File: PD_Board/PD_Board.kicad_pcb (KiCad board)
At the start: 2 copper layers, 116 x 63 mm, 12 parts

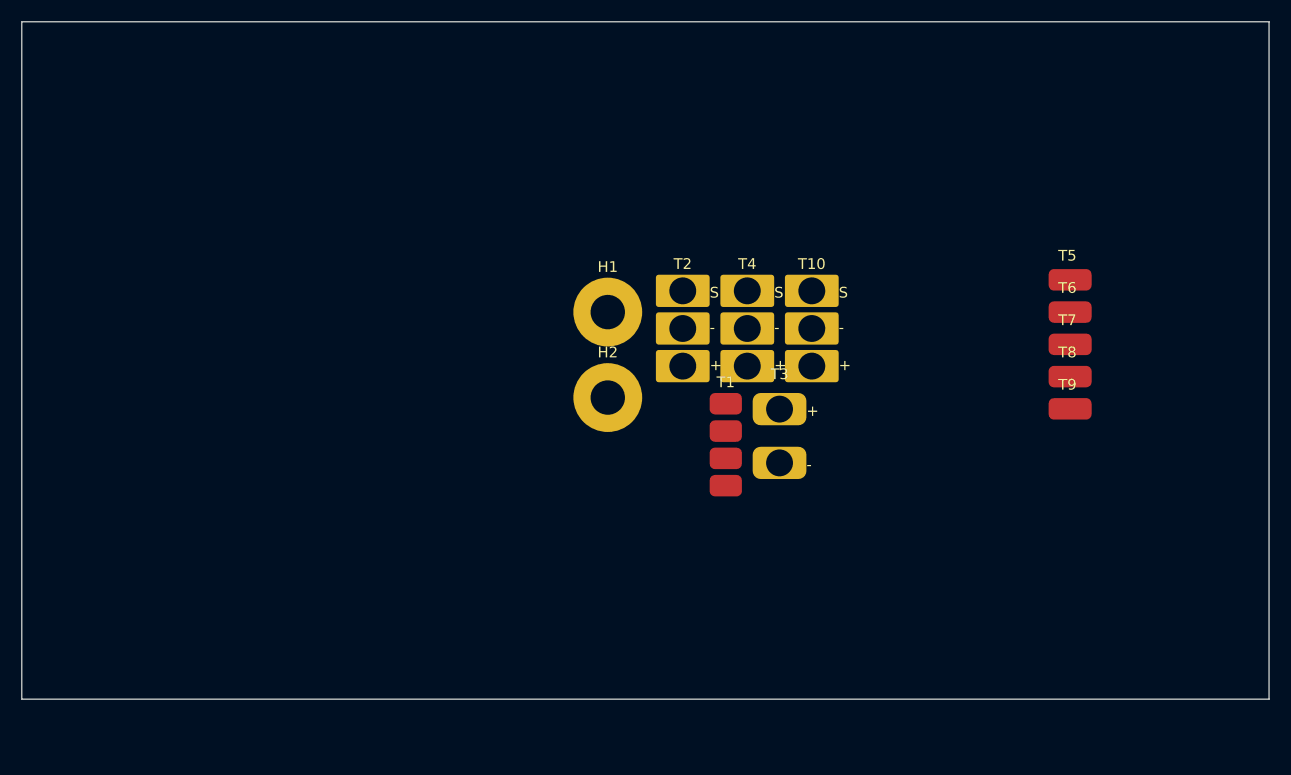
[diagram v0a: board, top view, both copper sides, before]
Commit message: womp womp
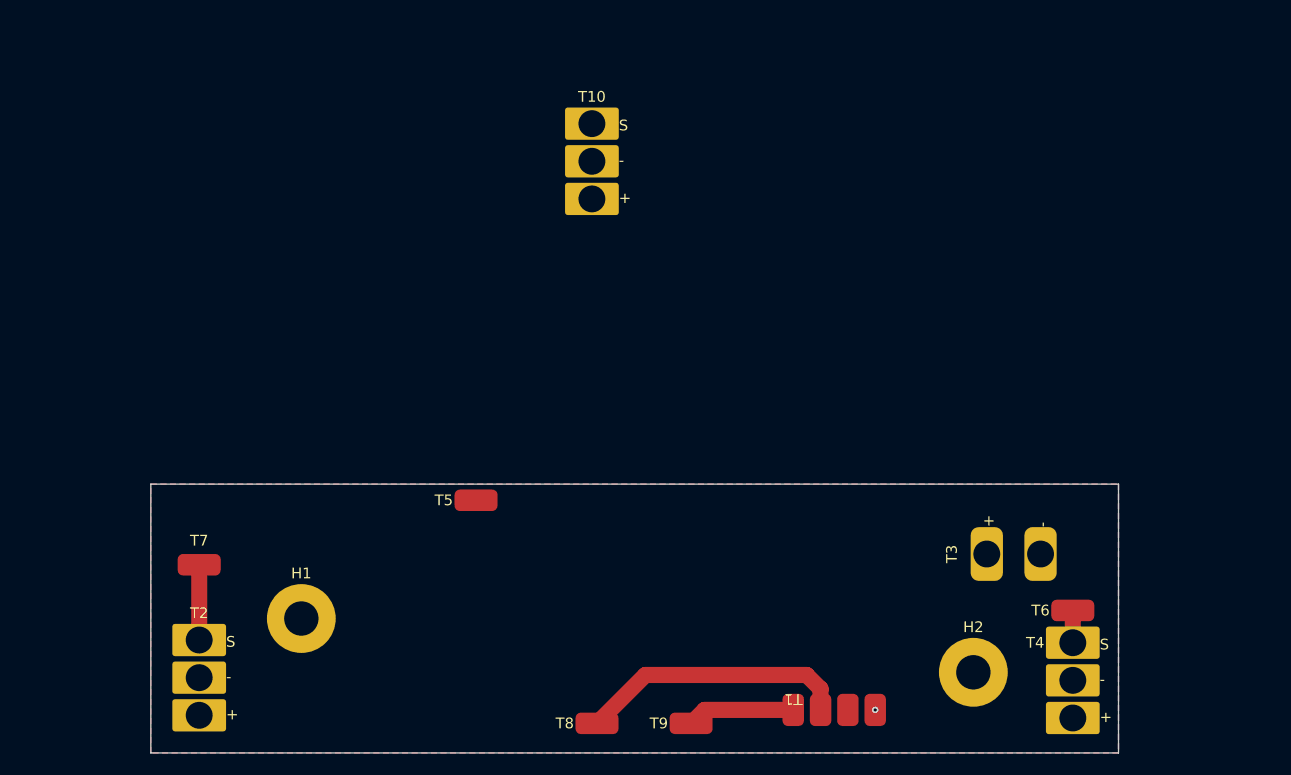
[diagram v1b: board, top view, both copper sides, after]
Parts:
- moved T7 83.6 mm to (104.5, 107.5), turned to 180 degrees
- moved T5 58.9 mm to (130.2, 101.5)
- moved T2 55.5 mm to (104.5, 114.5)
- moved T8 54.6 mm to (141.5, 122.2), turned to 180 degrees
- moved T9 45.8 mm to (150.2, 122.2), turned to 180 degrees
- moved T4 44.6 mm to (185.8, 114.8)
- moved H2 42.5 mm to (176.5, 117.5)
- moved H1 40.3 mm to (114.0, 112.5)
- moved T1 29.2 mm to (159.8, 121.0), turned to 90 degrees
- moved T6 27.8 mm to (185.8, 111.8), turned to 180 degrees
- moved T10 25.7 mm to (141.0, 66.5)
- moved T3 23.5 mm to (177.8, 106.5), turned to 90 degrees
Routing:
- net Net-(T1-Pad2): track 0.00 -> 25.1 mm
- net Net-(T1-Pad1): track 0.00 -> 10.0 mm
- net Net-(T2-Pad1): track 0.00 -> 7.00 mm
- net Net-(T4-Pad1): track 0.00 -> 3.00 mm
- net Net-(T3--): vias 0 -> 1
- added copper zone on F.Cu, net Net-(T3-+)
- added copper zone on B.Cu, net Net-(T3--)
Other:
- board size 116 x 63 mm -> 90 x 25 mm
